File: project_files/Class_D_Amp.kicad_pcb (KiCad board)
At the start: 2 copper layers, 90 x 100 mm, 87 parts, among them P1 ROUT, P2 LOUT, P3 CONN_01X04, P4 2x12V, Q1 BC847, Q2 BC857, Q3 IPD180N10, Q4 IPD180N10, Q5 IPD180N10, Q6 IPD180N10, U1 LM360, U2 UCC27201, U3 LM833, U4 IES101-4, U5 LM360, U6 UCC27201

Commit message: Generated Gerbers
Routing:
- net GND: track 66.9 -> 43.2 mm, vias 40 -> 28
- net (no net): track 0.00 -> 23.7 mm, vias 0 -> 12
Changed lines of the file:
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@@
     (links 176)
     (no_connects 0)
-    (area 19.924999 14.924999 110.075001 115.075001)
+    (area 14.342857 12.845 116.100001 119.125001)
     (thickness 1.6)
     (drawings 9)
@@
     (visible_elements FFFEFF7F)
     (pcbplotparams
-      (layerselection 0x00030_80000001)
+      (layerselection 0x010f0_80000001)
       (usegerberextensions false)
-      (excludeedgelayer true)
-      (linewidth 0.100000)
-      (plotframeref true)
+      (usegerberattributes true)
+      (excludeedgelayer false)
+      (linewidth 0.150000)
+      (plotframeref false)
       (viasonmask false)
       (mode 1)
-      (useauxorigin false)
+      (useauxorigin true)
       (hpglpennumber 1)
       (hpglpenspeed 20)
@@
       (padsonsilk false)
       (subtractmaskfromsilk false)
-      (outputformat 4)
+      (outputformat 1)
       (mirror false)
       (drillshape 0)
       (scaleselection 1)
-      (outputdirectory ""))
+      (outputdirectory plots/))
   )
   (net 0 "")
@@
   (gr_arc (start 105 20) (end 105 15) (angle 90) (layer Edge.Cuts) (width 0.15))
   (gr_arc (start 105 110) (end 110 110) (angle 90) (layer Edge.Cuts) (width 0.15))
+  (via (at 70.9 53.9) (size 0.6) (drill 0.4) (layers F.Cu B.Cu) (net 0))
+  (via (at 73.45 51.4) (size 0.6) (drill 0.4) (layers F.Cu B.Cu) (net 0))
+  (segment (start 73.45 51.4) (end 70.95 53.9) (width 0.3) (layer F.Cu) (net 0))
+  (segment (start 70.95 53.9) (end 70.9 53.9) (width 0.3) (layer F.Cu) (net 0))
+  (via (at 88.65 70) (size 0.6) (drill 0.4) (layers F.Cu B.Cu) (net 0))
+  (via (at 88.65 66.5) (size 0.6) (drill 0.4) (layers F.Cu B.Cu) (net 0))
+  (segment (start 88.65 70) (end 88.65 66.5) (width 0.3) (layer F.Cu) (net 0))
+  (via (at 53.5 46.75) (size 1) (drill 0.6) (layers F.Cu B.Cu) (net 0))
+  (via (at 49.25 46.75) (size 1) (drill 0.6) (layers F.Cu B.Cu) (net 0))
+  (segment (start 53.5 46.75) (end 49.25 46.75) (width 1.22) (layer F.Cu) (net 0))
+  (segment (start 53.75 53.5) (end 53.5 53.5) (width 1.22) (layer B.Cu) (net 0))
+  (via (at 49.5 53.5) (size 1) (drill 0.6) (layers F.Cu B.Cu) (net 0))
+  (segment (start 53.5 53.5) (end 49.5 53.5) (width 1.22) (layer F.Cu) (net 0))
+  (via (at 53.5 53.5) (size 1) (drill 0.6) (layers F.Cu B.Cu) (net 0))
+  (via (at 63.75 47) (size 1) (drill 0.6) (layers F.Cu B.Cu) (net 0))
+  (via (at 66.5 44.25) (size 1) (drill 0.6) (layers F.Cu B.Cu) (net 0))
+  (segment (start 63.75 47) (end 66.5 44.25) (width 1.22) (layer F.Cu) (net 0))
+  (via (at 67 50.75) (size 1) (drill 0.6) (layers F.Cu B.Cu) (net 0))
+  (via (at 70 47.75) (size 1) (drill 0.6) (layers F.Cu B.Cu) (net 0))
+  (segment (start 67 50.75) (end 70 47.75) (width 1.22) (layer F.Cu) (net 0))
   (segment (start 76.15 78.1) (end 76.15 77.9) (width 0.5) (layer F.Cu) (net 1))
   (segment (start 76.15 77.9) (end 75 76.75) (width 0.5) (layer F.Cu) (net 1))
@@
   (segment (start 62.55 86.45) (end 62.25 86.75) (width 0.5) (layer F.Cu) (net 1))
   (segment (start 62.25 86.75) (end 62.25 88.25) (width 0.5) (layer F.Cu) (net 1))
-  (via (at 70.9 53.9) (size 0.6) (drill 0.4) (layers F.Cu B.Cu) (net 2))
-  (via (at 73.45 51.4) (size 0.6) (drill 0.4) (layers F.Cu B.Cu) (net 2))
-  (segment (start 73.45 51.4) (end 70.95 53.9) (width 0.3) (layer F.Cu) (net 2))
-  (segment (start 70.95 53.9) (end 70.9 53.9) (width 0.3) (layer F.Cu) (net 2))
-  (via (at 88.65 70) (size 0.6) (drill 0.4) (layers F.Cu B.Cu) (net 2))
-  (via (at 88.65 66.5) (size 0.6) (drill 0.4) (layers F.Cu B.Cu) (net 2))
-  (segment (start 88.65 70) (end 88.65 66.5) (width 0.3) (layer F.Cu) (net 2))
-  (via (at 53.5 46.75) (size 1) (drill 0.6) (layers F.Cu B.Cu) (net 2))
-  (via (at 49.25 46.75) (size 1) (drill 0.6) (layers F.Cu B.Cu) (net 2))
-  (segment (start 53.5 46.75) (end 49.25 46.75) (width 1.22) (layer F.Cu) (net 2))
-  (segment (start 53.75 53.5) (end 53.5 53.5) (width 1.22) (layer B.Cu) (net 2))
-  (via (at 49.5 53.5) (size 1) (drill 0.6) (layers F.Cu B.Cu) (net 2))
-  (segment (start 53.5 53.5) (end 49.5 53.5) (width 1.22) (layer F.Cu) (net 2))
-  (via (at 53.5 53.5) (size 1) (drill 0.6) (layers F.Cu B.Cu) (net 2))
-  (via (at 63.75 47) (size 1) (drill 0.6) (layers F.Cu B.Cu) (net 2))
-  (via (at 66.5 44.25) (size 1) (drill 0.6) (layers F.Cu B.Cu) (net 2))
-  (segment (start 63.75 47) (end 66.5 44.25) (width 1.22) (layer F.Cu) (net 2))
-  (via (at 67 50.75) (size 1) (drill 0.6) (layers F.Cu B.Cu) (net 2))
-  (via (at 70 47.75) (size 1) (drill 0.6) (layers F.Cu B.Cu) (net 2))
-  (segment (start 67 50.75) (end 70 47.75) (width 1.22) (layer F.Cu) (net 2))
   (segment (start 55 80.5) (end 55 82) (width 0.5) (layer F.Cu) (net 2))
   (via (at 55 82) (size 1) (drill 0.6) (layers F.Cu B.Cu) (net 2))

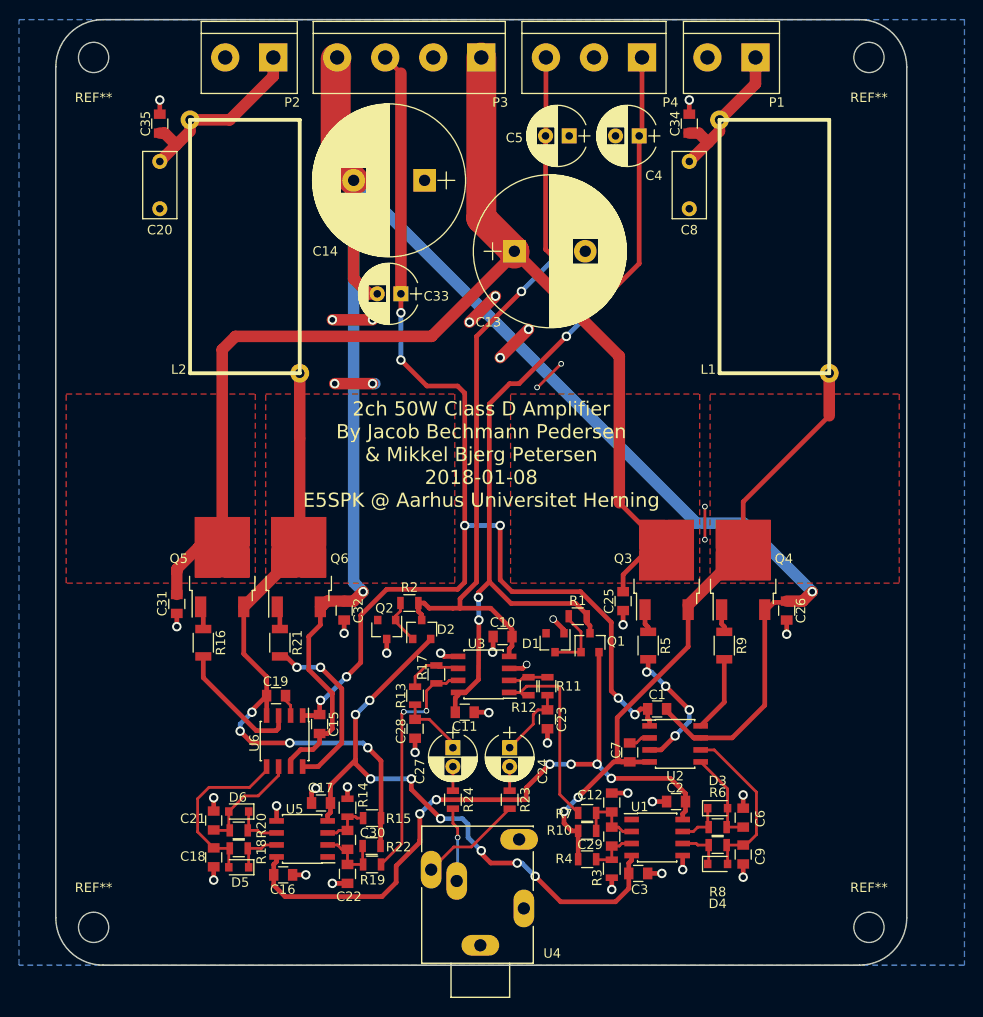
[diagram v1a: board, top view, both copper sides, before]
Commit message: fixed size
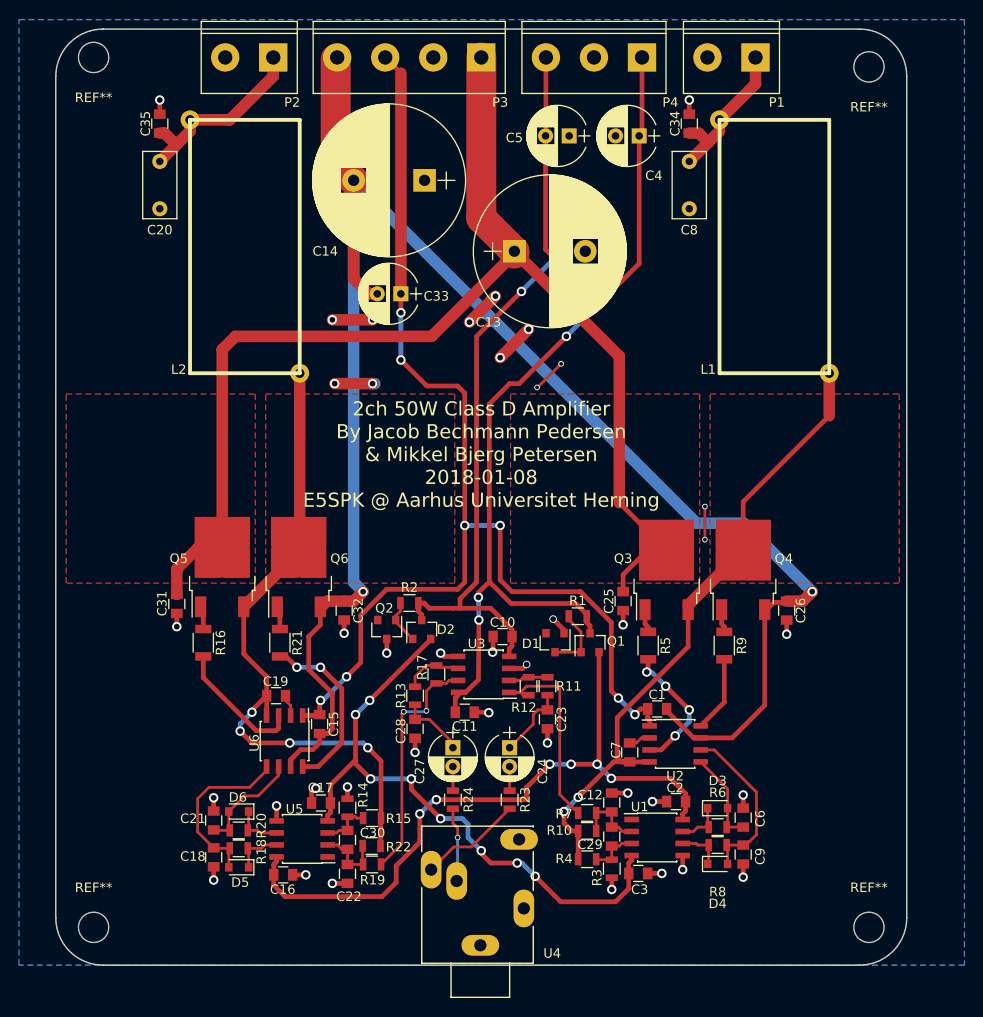
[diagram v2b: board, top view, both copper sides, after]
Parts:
- moved REF** 1.00 mm to (106.0, 20.0)
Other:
- board size 90 x 100 mm -> 90 x 99 mm
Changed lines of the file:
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@@
   )
   (module Mounting_Holes:MountingHole_3.2mm_M3 (layer F.Cu)
-    (at 106 19)
+    (at 106 20)
     (descr "Mounting Hole 3.2mm, no annular, M3")
     (tags "mounting hole 3.2mm no annular m3")
@@
     (pad 1 np_thru_hole circle (at 0 0) (size 3.2 3.2) (drill 3.2) (layers *.Cu *.Mask))
   )
+  (gr_line (start 110 21) (end 110 110) (angle 90) (layer Edge.Cuts) (width 0.15))
+  (gr_line (start 20 21) (end 20 110) (angle 90) (layer Edge.Cuts) (width 0.15))
   (gr_text "2ch 50W Class D Amplifier\nBy Jacob Bechmann Pedersen\n& Mikkel Bjerg Petersen\n2018-01-08\nE5SPK @ Aarhus Universitet Herning" (at 65 61) (layer F.SilkS)
     (effects (font (size 1.5 1.5) (thickness 0.3)))
   )
-  (gr_line (start 105 15) (end 25 15) (angle 90) (layer Edge.Cuts) (width 0.15))
+  (gr_line (start 105 16) (end 25 16) (angle 90) (layer Edge.Cuts) (width 0.15))
   (gr_line (start 25 115) (end 105 115) (angle 90) (layer Edge.Cuts) (width 0.15))
-  (gr_line (start 110 110) (end 110 20) (angle 90) (layer Edge.Cuts) (width 0.15))
-  (gr_line (start 20 110) (end 20 20) (angle 90) (layer Edge.Cuts) (width 0.15))
   (gr_arc (start 25 110) (end 25 115) (angle 90) (layer Edge.Cuts) (width 0.15))
-  (gr_arc (start 25 20) (end 20 20) (angle 90) (layer Edge.Cuts) (width 0.15))
-  (gr_arc (start 105 20) (end 105 15) (angle 90) (layer Edge.Cuts) (width 0.15))
+  (gr_arc (start 25 21) (end 20 21) (angle 90) (layer Edge.Cuts) (width 0.15))
+  (gr_arc (start 105 21) (end 105 16) (angle 90) (layer Edge.Cuts) (width 0.15))
   (gr_arc (start 105 110) (end 110 110) (angle 90) (layer Edge.Cuts) (width 0.15))
   (via (at 70.9 53.9) (size 0.6) (drill 0.4) (layers F.Cu B.Cu) (net 0))
